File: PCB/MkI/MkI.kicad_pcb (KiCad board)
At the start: 2 copper layers, 24.8 x 20.8 mm, 10 parts, among them J1 Conn_RX, J2 Conn_TX, U1 CH32V003FxPx

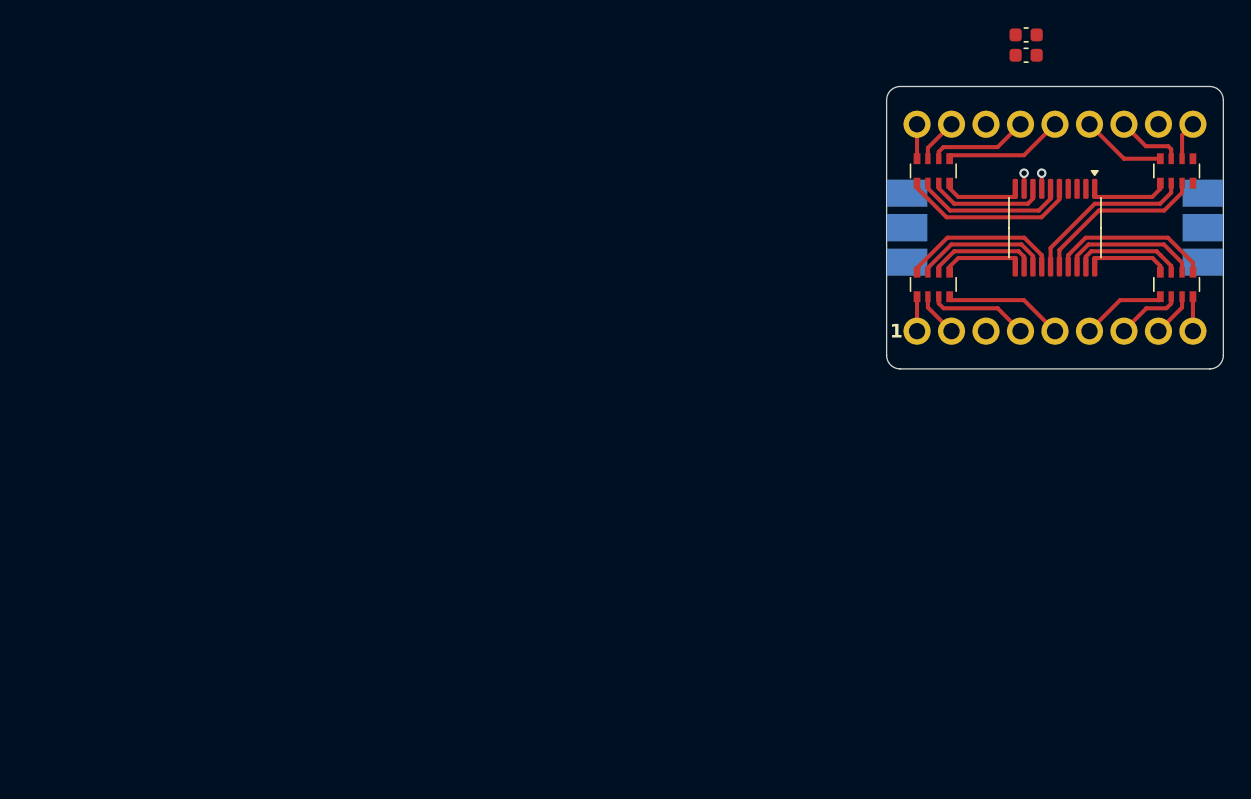
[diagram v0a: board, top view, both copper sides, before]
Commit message: MkI PCB Finished
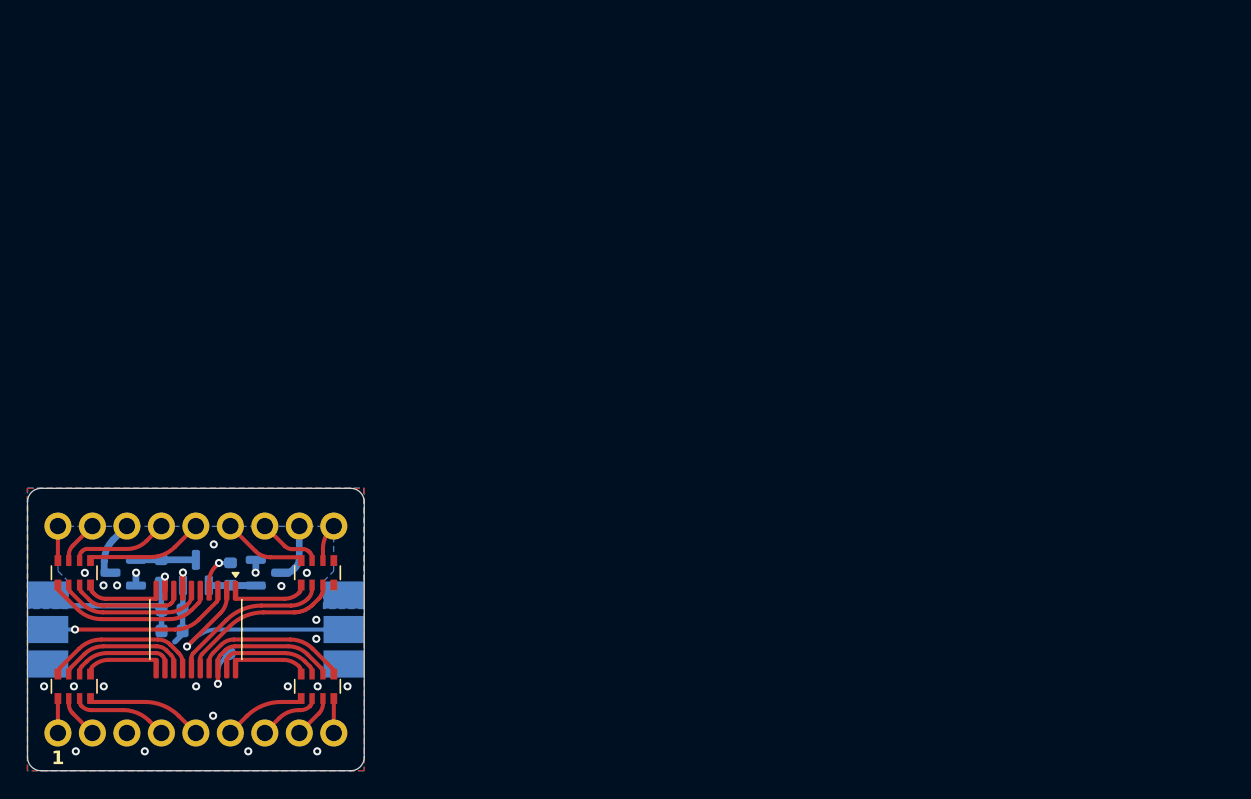
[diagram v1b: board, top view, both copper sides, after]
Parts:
- added Q1: AO3400A, Project_Footprints:SOT-23_Clean, B.Cu at (93.1, 82.8)
- added Q2: AO3400A, Project_Footprints:SOT-23_Clean, B.Cu at (103.8, 82.8)
- added Q3: AO3400A, Project_Footprints:SOT-23_Clean, B.Cu at (98.4, 82.8)
- added R1: 10R, Resistor_SMD:R_0603_1608Metric, B.Cu at (101.0, 82.9)
- added R2: 2K2, Resistor_SMD:R_0603_1608Metric, B.Cu at (95.9, 82.7)
- added TP1: SWIO, TestPoint:TestPoint_Pad_D1.0mm, B.Cu at (100.9, 88.7)
- C1, C2: moved to B.Cu
- moved C2 75.9 mm to (96.7, 87.1)
- moved C1 75.8 mm to (96.7, 85.5)
- moved J1 69.9 mm to (87.5, 87.0)
- moved RN1 69.9 mm to (89.5, 91.2)
- moved RN3 69.9 mm to (89.5, 82.8)
- moved DISP1 69.9 mm to (98.4, 87.0)
- moved J2 69.9 mm to (109.3, 87.0)
- moved RN2 69.9 mm to (107.4, 91.2)
- moved RN4 69.9 mm to (107.4, 82.8)
- moved U1 69.9 mm to (98.4, 87.0)
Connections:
- DISP1 pad 11: unconnected-(DISP1-DIGIT_2-Pad11) -> /DIGIT_2
- DISP1 pad 16: unconnected-(DISP1-DIGIT_1-Pad16) -> /DIGIT_1
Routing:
- net /GPIO_PD5: track 0.00 -> 17.2 mm, vias 0 -> 1
- net /GPIO_PD6: track 0.00 -> 14.0 mm, vias 0 -> 1
- net VCC: track 1.15 -> 14.4 mm
- net GND: track 1.15 -> 9.41 mm, vias 1 -> 23
- net /DIGIT_1: track 0.00 -> 4.48 mm
- net Net-(Q1-G): track 0.00 -> 4.42 mm
- net /DIGIT_2: track 0.00 -> 4.30 mm
- net Net-(Q2-G): track 0.00 -> 3.47 mm
- net /GPIO_PD1: track 10.1 -> 13.4 mm, vias 0 -> 1
- net /GPIO_PD7: track 0.00 -> 3.12 mm, vias 0 -> 1
- net /GPIO_PC5: track 12.6 -> 12.1 mm
- added copper zone on B.Cu, net GND
- added copper zone on F.Cu, net GND
- added copper zone on B.Cu, net VCC
